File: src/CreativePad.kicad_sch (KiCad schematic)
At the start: 65 parts, among them SW2 TS342A2P-WZ, U1 TPMIC5219-2.8YM5, U17 RP2040_C2961140, U19 W25Q128JWPIQ, U2 AMS1117-3.3, X2 DSX321G-12MHZ

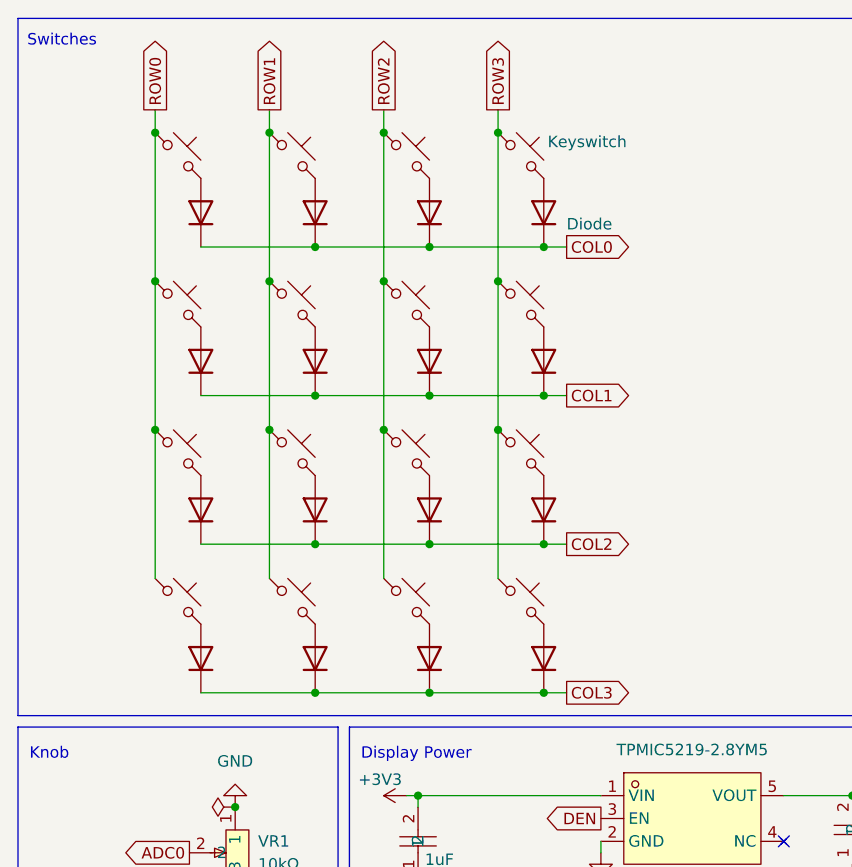
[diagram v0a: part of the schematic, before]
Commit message: Day 5
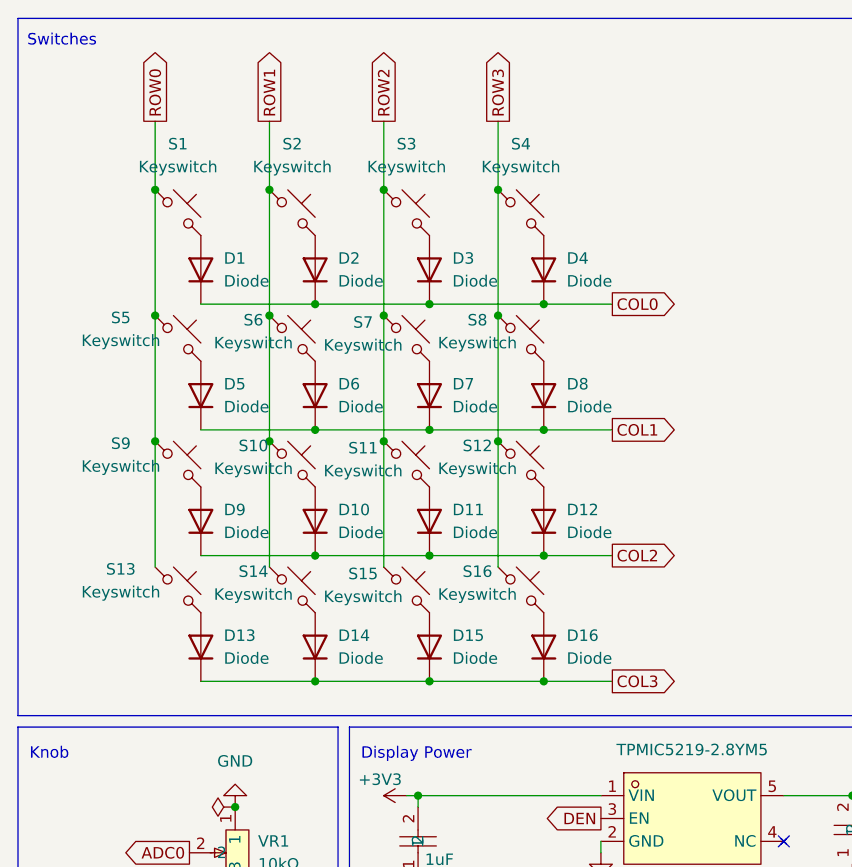
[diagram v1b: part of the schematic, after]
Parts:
- S1, S10, S11, S12, S13, S14, S15, S16, S2, S3, S4, S5, S6, S7, S8, S9: footprint ScottoKeebs_Scotto:MX_Hotswap_1.00u -> Switch_Keyboard_Hotswap_Kailh:SW_Hotswap_Kailh_MX_1.00u

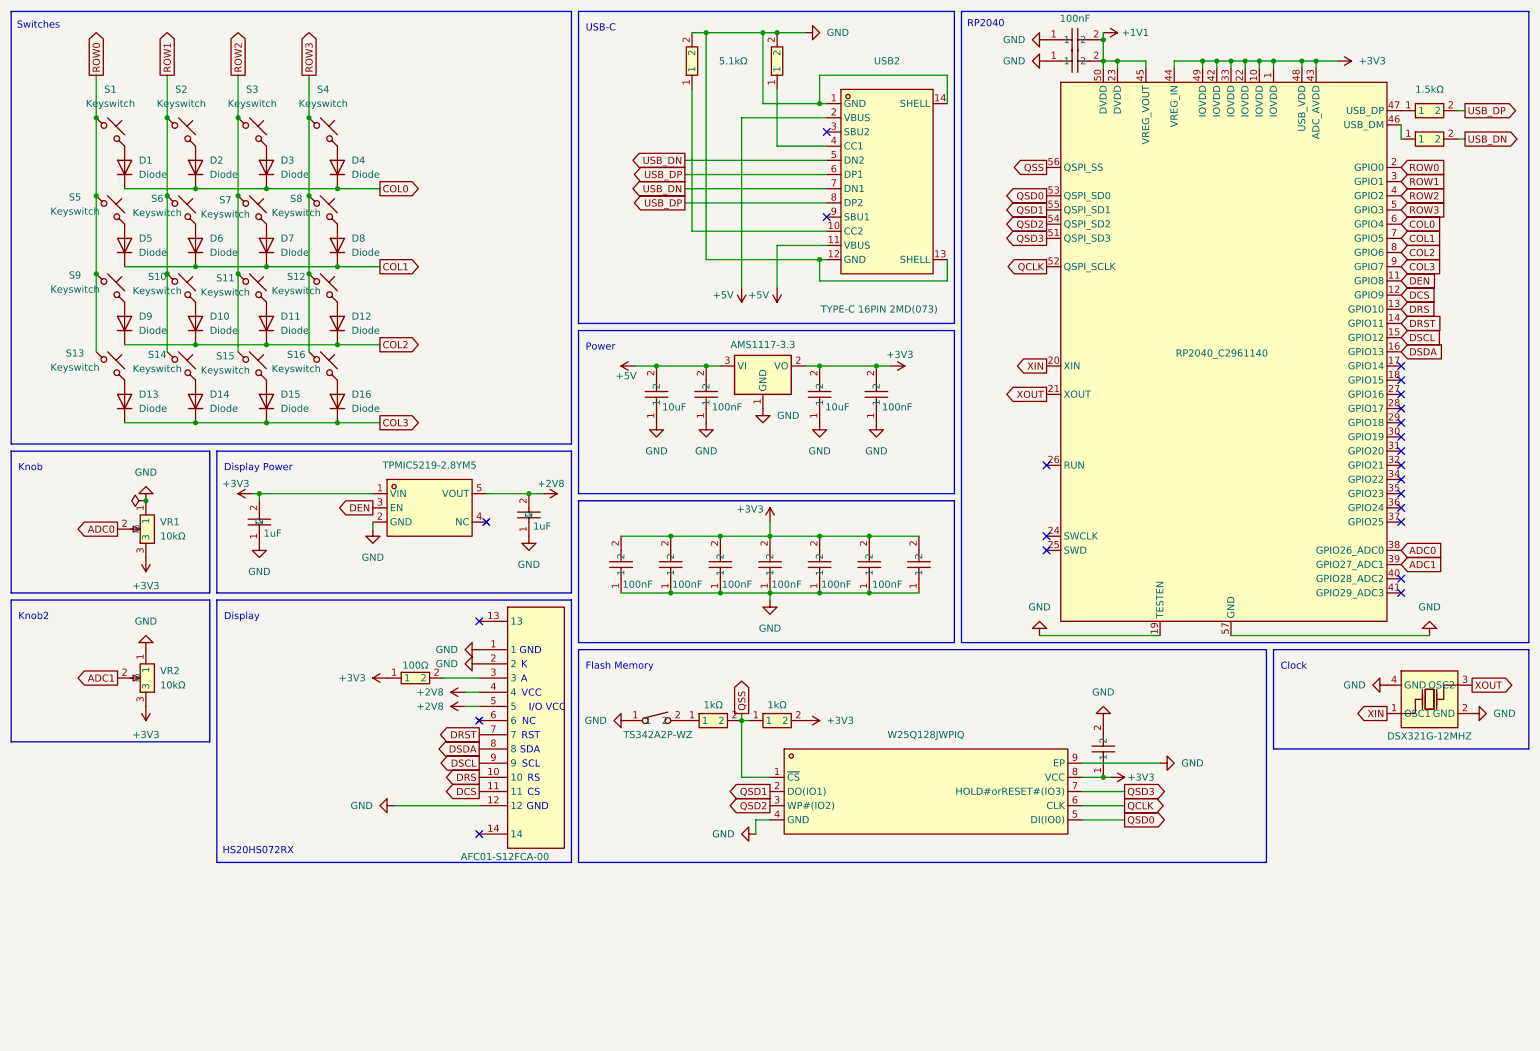
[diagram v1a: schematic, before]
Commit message: Day 6
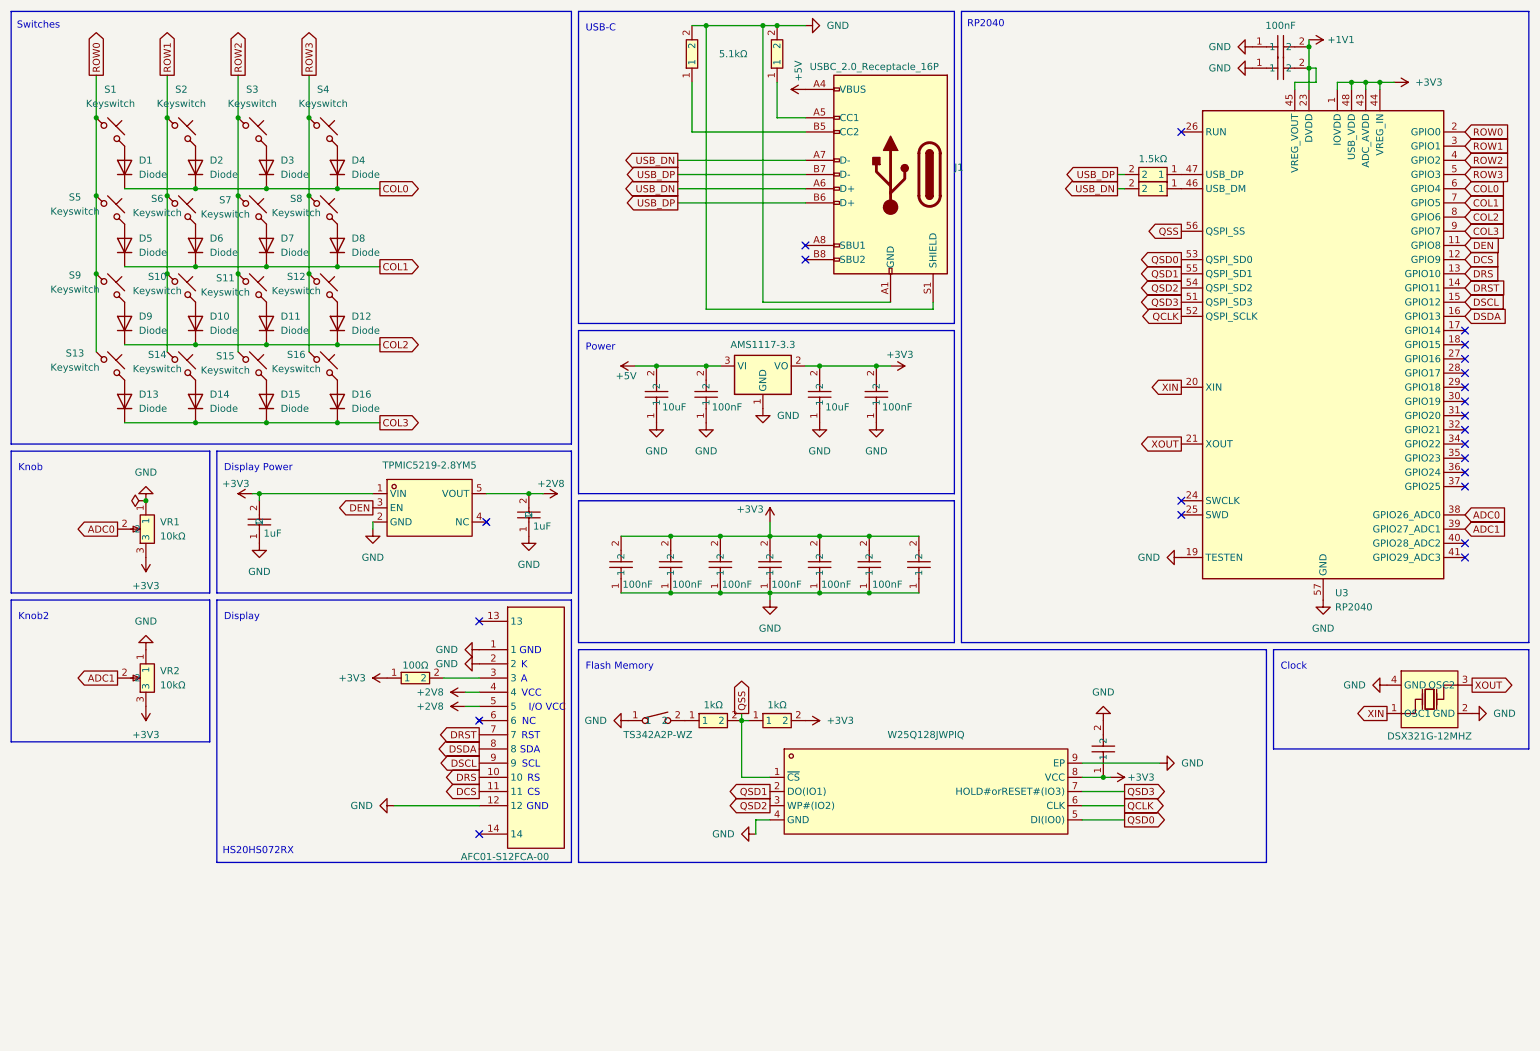
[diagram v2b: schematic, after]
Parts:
- removed C13, C17: 100nF, easyeda2kicad:C0603, symbol easyeda2kicad:CC0603KRX7R9BB104
- removed R1, R6: 5.1kΩ, easyeda2kicad:R0603, symbol easyeda2kicad:RC0603FR-075K1L
- removed R5, R7: 1.5kΩ, easyeda2kicad:R0603, symbol easyeda2kicad:FRC0603J152TS
- removed U17: RP2040_C2961140, easyeda2kicad:QFN-56_L7.0-W7.0-P0.40-TL-EP4.0, symbol easyeda2kicad:RP2040_C2961140
- removed USB2: TYPE-C 16PIN 2MD(073), easyeda2kicad:USB-C-SMD_TYPE-C-6PIN-2MD-073, symbol easyeda2kicad:TYPE-C16PIN2MD(073)
- added C16, C18: 100nF, easyeda2kicad:C0603, symbol easyeda2kicad:CC0603KRX7R9BB104
- added J1: USBC_2.0_Receptacle_16P, symbol Connector:USB_C_Receptacle_USB2.0_16P
- added R1, R6: 1.5kΩ, easyeda2kicad:R0603, symbol easyeda2kicad:FRC0603J152TS
- added R4, R9: 5.1kΩ, easyeda2kicad:R0603, symbol easyeda2kicad:RC0603FR-075K1L
- added U3: RP2040, Package_DFN_QFN:QFN-56-1EP_7x7mm_P0.4mm_EP3.2x3.2mm, symbol MCU_RaspberryPi:RP2040
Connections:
- net +1V1: now also C16.2, C18.2, U3.23 (DVDD), U3.45 (VREG_VOUT), U3.50 (DVDD)
- net +3V3: now also U3.1 (IOVDD), U3.10 (IOVDD), U3.22 (IOVDD), U3.33 (IOVDD), U3.42 (IOVDD), U3.43 (ADC_AVDD), U3.44 (VREG_IN), U3.48 (USB_VDD), U3.49 (IOVDD)
- net +5V: now also J1.A4 (VBUS), J1.A9 (VBUS), J1.B4 (VBUS), J1.B9 (VBUS)
- net ADC0: now also U3.38 (GPIO26_ADC0)
- net ADC1: now also U3.39 (GPIO27_ADC1)
- net COL0: now also U3.6 (GPIO4)
- net COL1: now also U3.7 (GPIO5)
- net COL2: now also U3.8 (GPIO6)
- net COL3: now also U3.9 (GPIO7)
- net DCS: now also U3.12 (GPIO9)
- net DEN: now also U3.11 (GPIO8)
- net DRS: now also U3.13 (GPIO10)
- net DRST: now also U3.14 (GPIO11)
- net DSCL: now also U3.15 (GPIO12)
- net DSDA: now also U3.16 (GPIO13)
- net GND: now also C16.1, C18.1, J1.A1 (GND), J1.A12 (GND), J1.B1 (GND), J1.B12 (GND), J1.S1 (SHIELD), R4.2, R9.2, U3.19 (TESTEN), U3.57 (GND)
- net QCLK: now also U3.52 (QSPI_SCLK)
- net QSD0: now also U3.53 (QSPI_SD0)
- net QSD1: now also U3.55 (QSPI_SD1)
- net QSD2: now also U3.54 (QSPI_SD2)
- net QSD3: now also U3.51 (QSPI_SD3)
- net QSS: now also U3.56 (QSPI_SS)
- net ROW0: now also U3.2 (GPIO0)
- net ROW1: now also U3.3 (GPIO1)
- net ROW2: now also U3.4 (GPIO2)
- net ROW3: now also U3.5 (GPIO3)
- net USB_DN: now also J1.A6 (D+), J1.A7 (D-), R6.2
- net USB_DP: now also J1.B6 (D+), J1.B7 (D-), R1.2
- net XIN: now also U3.20 (XIN)
- net XOUT: now also U3.21 (XOUT)
- new net: J1.A5 (CC1), R9.1
- new net: J1.B5 (CC2), R4.1
- new net: R6.1, U3.46 (USB_DM)
- new net: R1.1, U3.47 (USB_DP)

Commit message: Day 8
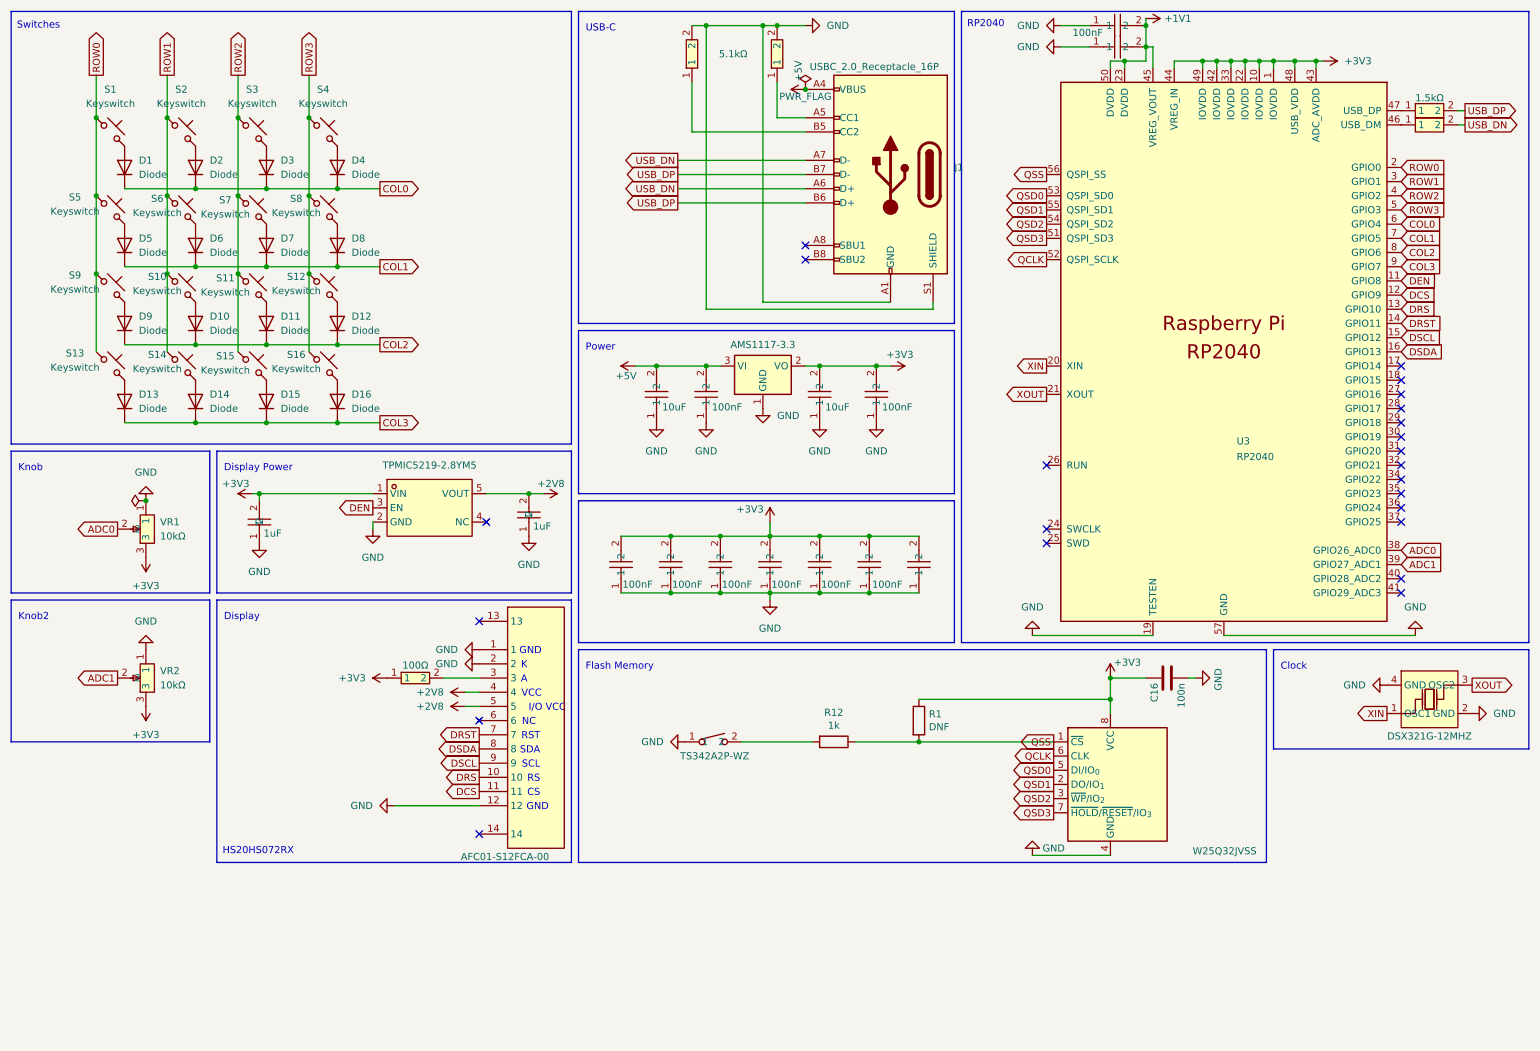
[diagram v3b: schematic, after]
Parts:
- removed C11, C16, C18: 100nF, easyeda2kicad:C0603, symbol easyeda2kicad:CC0603KRX7R9BB104
- removed R1: 1.5kΩ, easyeda2kicad:R0603, symbol easyeda2kicad:FRC0603J152TS
- removed R2, R3: 1kΩ, easyeda2kicad:R0402, symbol easyeda2kicad:FRC0402J102TS
- removed SW2: TS342A2P-WZ, easyeda2kicad:SW-SMD_L4.0-W2.9-LS5.0, symbol easyeda2kicad:TS342A2P-WZ
- removed U19: W25Q128JWPIQ, easyeda2kicad:WSON-8_L6.0-W5.0-P1.27-BL-EP, symbol easyeda2kicad:W25Q128JWPIQ
- removed U3: RP2040, Package_DFN_QFN:QFN-56-1EP_7x7mm_P0.4mm_EP3.2x3.2mm, symbol MCU_RaspberryPi:RP2040
- added C13, C17: 100nF, easyeda2kicad:C0603, symbol easyeda2kicad:CC0603KRX7R9BB104
- added C16: 100n, Capacitor_SMD:C_0402_1005Metric, symbol Device:C
- added R1: DNF, Resistor_SMD:R_0402_1005Metric, symbol Device:R
- added R12: 1k, Resistor_SMD:R_0402_1005Metric, symbol Device:R
- added R2: 1.5kΩ, easyeda2kicad:R0603, symbol easyeda2kicad:FRC0603J152TS
- added SW1: TS342A2P-WZ, easyeda2kicad:SW-SMD_L4.0-W2.9-LS5.0, symbol easyeda2kicad:TS342A2P-WZ
- added U3: RP2040, RP2040_minimal_r2:RP2040-QFN-56, symbol MCU_RaspberryPi_RP20401:RP2040
- added U5: W25Q32JVSS, Package_SO:SOIC-8_5.3x5.3mm_P1.27mm, symbol Memory_Flash:W25Q32JVSS
- J1: footprint (none) -> Connector_USB:USB_C_Receptacle_GCT_USB4110
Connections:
- net +1V1: now also C13.2, C17.2, U3.23 (DVDD), U3.45 (VREG_VOUT), U3.50 (DVDD)
- net +3V3: now also C16.1, R1.1, U3.1 (IOVDD), U3.10 (IOVDD), U3.22 (IOVDD), U3.33 (IOVDD), U3.42 (IOVDD), U3.43 (ADC_AVDD), U3.44 (VREG_IN), U3.48 (USB_VDD), U3.49 (IOVDD), U5.8 (VCC)
- net ADC0: now also U3.38 (GPIO26_ADC0)
- net ADC1: now also U3.39 (GPIO27_ADC1)
- net COL0: now also U3.6 (GPIO4)
- net COL1: now also U3.7 (GPIO5)
- net COL2: now also U3.8 (GPIO6)
- net COL3: now also U3.9 (GPIO7)
- net DCS: now also U3.12 (GPIO9)
- net DEN: now also U3.11 (GPIO8)
- net DRS: now also U3.13 (GPIO10)
- net DRST: now also U3.14 (GPIO11)
- net DSCL: now also U3.15 (GPIO12)
- net DSDA: now also U3.16 (GPIO13)
- net GND: now also C13.1, C16.2, C17.1, SW1.1, U3.19 (TESTEN), U3.57 (GND), U5.4 (GND)
- net QCLK: now also U3.52 (QSPI_SCLK), U5.6 (CLK)
- net QSD0: now also U3.53 (QSPI_SD0), U5.5 (DI/IO_{0})
- net QSD1: now also U3.55 (QSPI_SD1), U5.2 (DO/IO_{1})
- net QSD2: now also U3.54 (QSPI_SD2), U5.3 (~{WP}/IO_{2})
- net QSD3: now also U3.51 (QSPI_SD3), U5.7 (~{HOLD}/~{RESET}/IO_{3})
- net QSS: now also R1.2, R12.1, U3.56 (QSPI_SS), U5.1 (~{CS})
- net ROW0: now also U3.2 (GPIO0)
- net ROW1: now also U3.3 (GPIO1)
- net ROW2: now also U3.4 (GPIO2)
- net ROW3: now also U3.5 (GPIO3)
- net USB_DP: now also R2.2
- net XIN: now also U3.20 (XIN)
- net XOUT: now also U3.21 (XOUT)
- net at R6.1: now also U3.46 (USB_DM)
- new net: R12.2, SW1.2
- new net: R2.1, U3.47 (USB_DP)

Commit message: Day 8 - Part 2
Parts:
- J1: footprint Connector_USB:USB_C_Receptacle_GCT_USB4110 -> Connector_USB:USB_C_Receptacle_HCTL_HC-TYPE-C-16P-01A
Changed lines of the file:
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@@
 			)
 		)
-		(property "Footprint" "Connector_USB:USB_C_Receptacle_GCT_USB4110"
+		(property "Footprint" "Connector_USB:USB_C_Receptacle_HCTL_HC-TYPE-C-16P-01A"
 			(at 166.37 41.91 0)
 			(effects

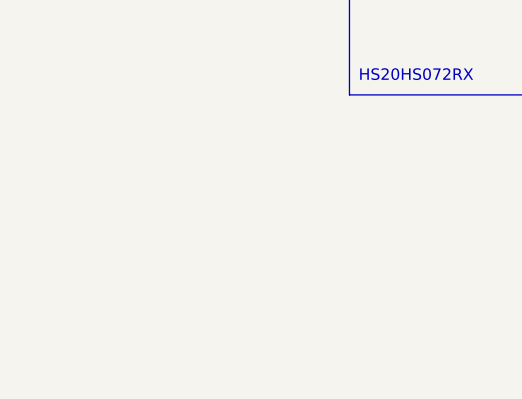
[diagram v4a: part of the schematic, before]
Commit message: Day 9
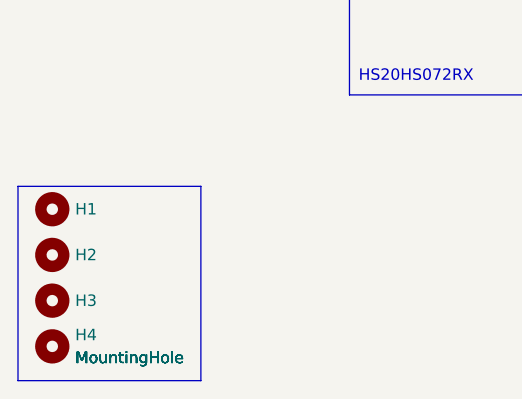
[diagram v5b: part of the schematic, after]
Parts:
- added H1, H2, H3, H4: MountingHole, MountingHole:MountingHole_2.2mm_M2, symbol Mechanical:MountingHole
